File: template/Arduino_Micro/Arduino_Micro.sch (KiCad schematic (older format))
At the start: 6 parts, among them P1 Digital, P2 Analog, P3 CONN_1, P4 CONN_1, P5 CONN_1, P6 CONN_1

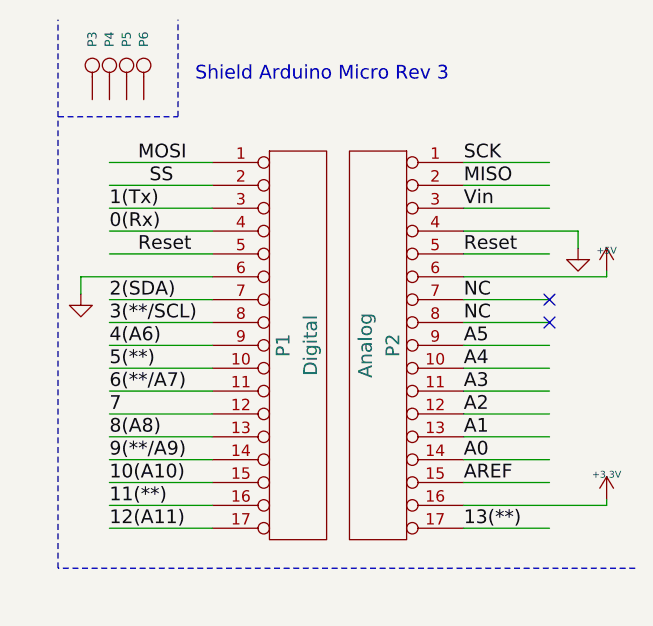
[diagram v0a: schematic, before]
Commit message: Correction schématics
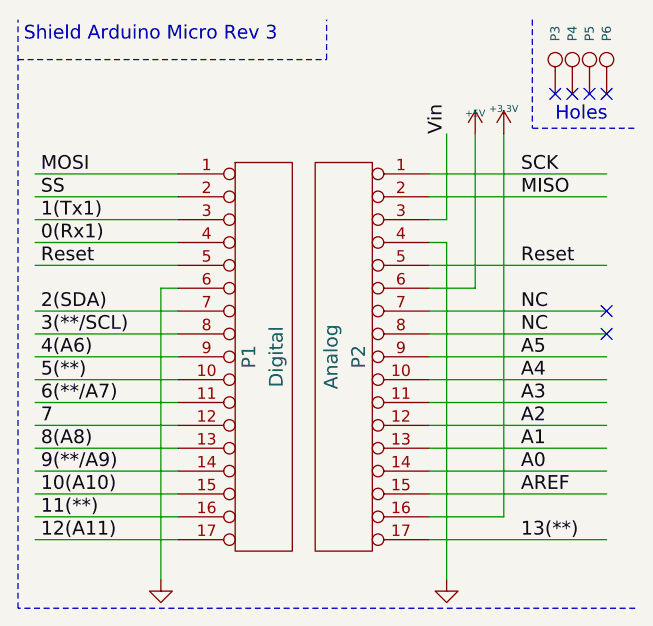
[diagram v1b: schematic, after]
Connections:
- net labels added: 0(Rx1), 1(Tx1)
- net labels removed: 0(Rx), 1(Tx)
- wire segments 38 -> 39
- no-connect marks 2 -> 6
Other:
- note added: "Holes"
- moved on the sheet: P1, P2, P3, P4, P5, P6
